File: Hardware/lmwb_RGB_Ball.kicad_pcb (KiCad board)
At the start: 2 copper layers, 65 x 65 mm, 41 parts, among them J1 Conn_01x03, J2 Conn_01x03, U1 AMS1117-3.3, U2 24C02S, U3 STM32C011F6P6

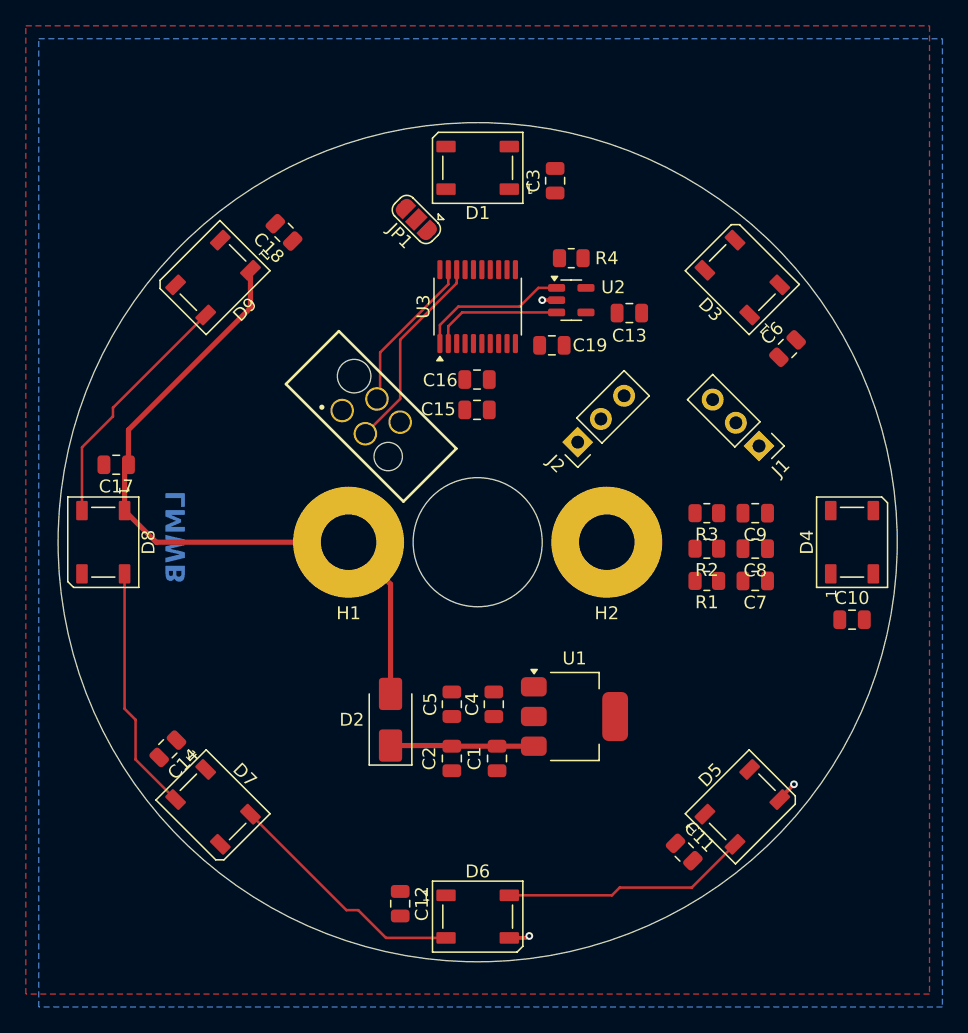
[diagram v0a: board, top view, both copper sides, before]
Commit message: progress on layout
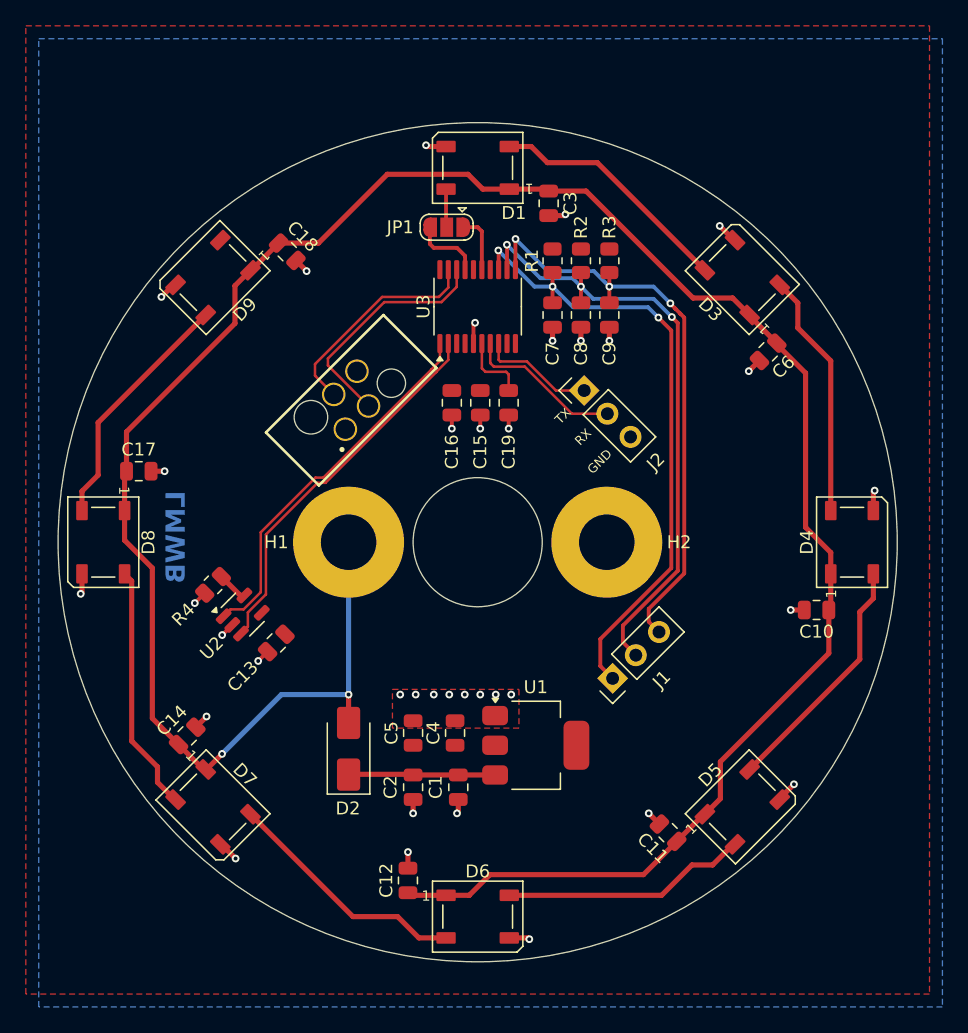
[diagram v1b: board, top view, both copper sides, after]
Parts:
- moved R4 37.6 mm to (49.5, 73.3), turned to 45 degrees
- moved C13 37.4 mm to (54.4, 77.8), turned to -135 degrees
- moved U2 35.2 mm to (51.8, 75.6), turned to 45 degrees
- moved R1 27.5 mm to (75.8, 48.2), turned to 90 degrees
- moved C7 25.9 mm to (75.8, 52.4), turned to -90 degrees
- moved R2 24.3 mm to (78.0, 48.2), turned to 90 degrees
- moved C8 22.6 mm to (78.0, 52.4), turned to -90 degrees
- moved J1 21.3 mm to (80.5, 80.5), turned to 135 degrees
- moved R3 21.0 mm to (80.2, 48.2), turned to 90 degrees
- moved C9 19.1 mm to (80.2, 52.4), turned to -90 degrees
- moved C19 5.57 mm to (72.4, 59.2), turned to -90 degrees
- moved J2 4.03 mm to (78.2, 58.2), turned to 45 degrees
- moved D2 3.95 mm to (60.0, 86.0)
- moved C1 3.74 mm to (68.5, 89.0)
- moved C2 3.74 mm to (65.0, 89.0)
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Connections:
- J2 pad 1: /UART-TX -> /UART-RX
- J2 pad 2: /UART-RX -> /UART-TX
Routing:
- net +5V: track 54.1 -> 190.2 mm, vias 0 -> 2
- net /EXTI-6: track 0.00 -> 49.4 mm, vias 0 -> 3
- net /EXTI-5: track 0.00 -> 47.9 mm, vias 0 -> 3
- net /EXTI-4: track 0.00 -> 46.1 mm, vias 0 -> 3
- net GND: track 4.36 -> 35.7 mm, vias 3 -> 36
- net /SDA: track 10.2 -> 29.5 mm
- net Net-(D3-DOUT): track 0.00 -> 19.1 mm
- net Net-(D4-DOUT): track 0.00 -> 19.1 mm
- net Net-(D1-DOUT): track 0.00 -> 19.1 mm
- net /SCL: track 11.7 -> 29.0 mm
- net /UART-TX: track 0.00 -> 12.2 mm
- net /UART-RX: track 0.00 -> 8.87 mm
- net /SPI-MOSI: track 0.00 -> 5.47 mm
- net /nRST: track 0.00 -> 5.43 mm
- net /SW-CLK: track 12.3 -> 17.1 mm
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- added copper zone on F.Cu, net GND
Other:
- board text added: "TX RX GND"
